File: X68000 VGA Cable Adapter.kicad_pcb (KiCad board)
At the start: 2 copper layers, 40.5 x 30.4 mm, 8 parts, among them J1 DE15_Receptacle_HighDensity, J2 DA15_Plug

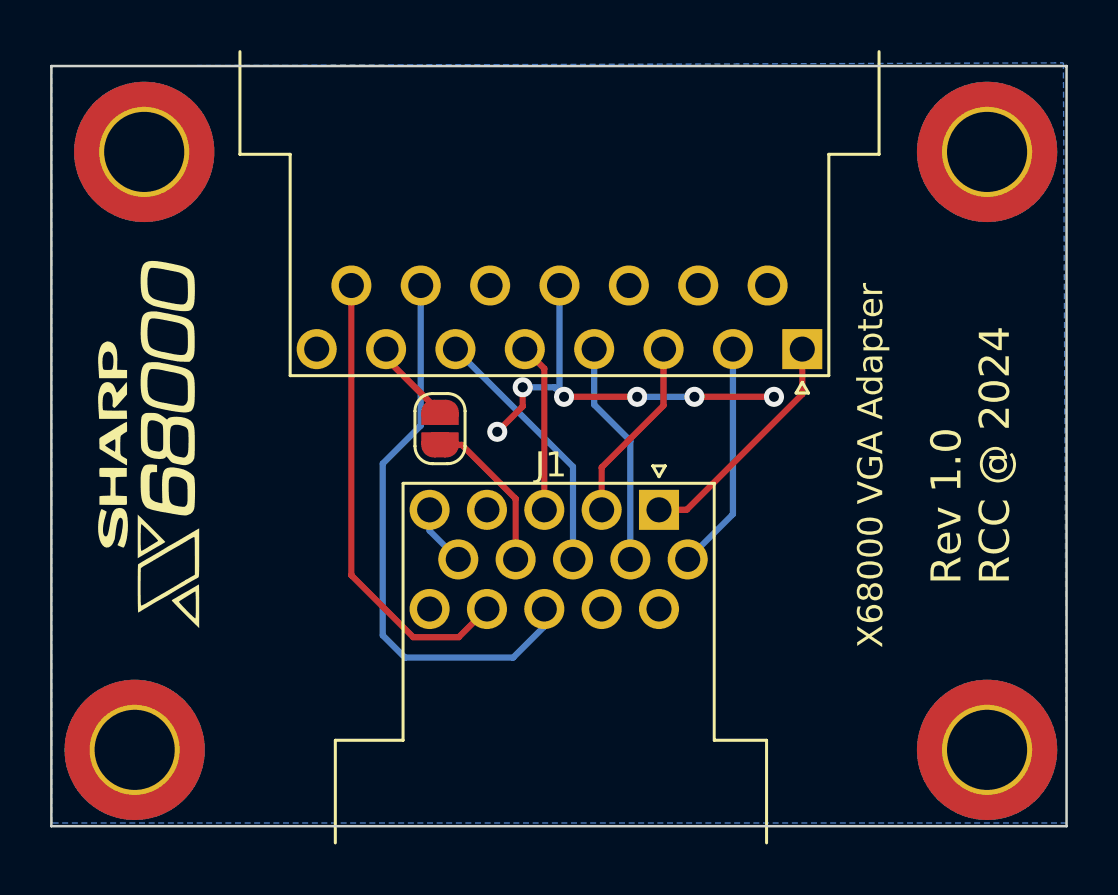
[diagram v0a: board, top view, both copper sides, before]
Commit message: Fabricated
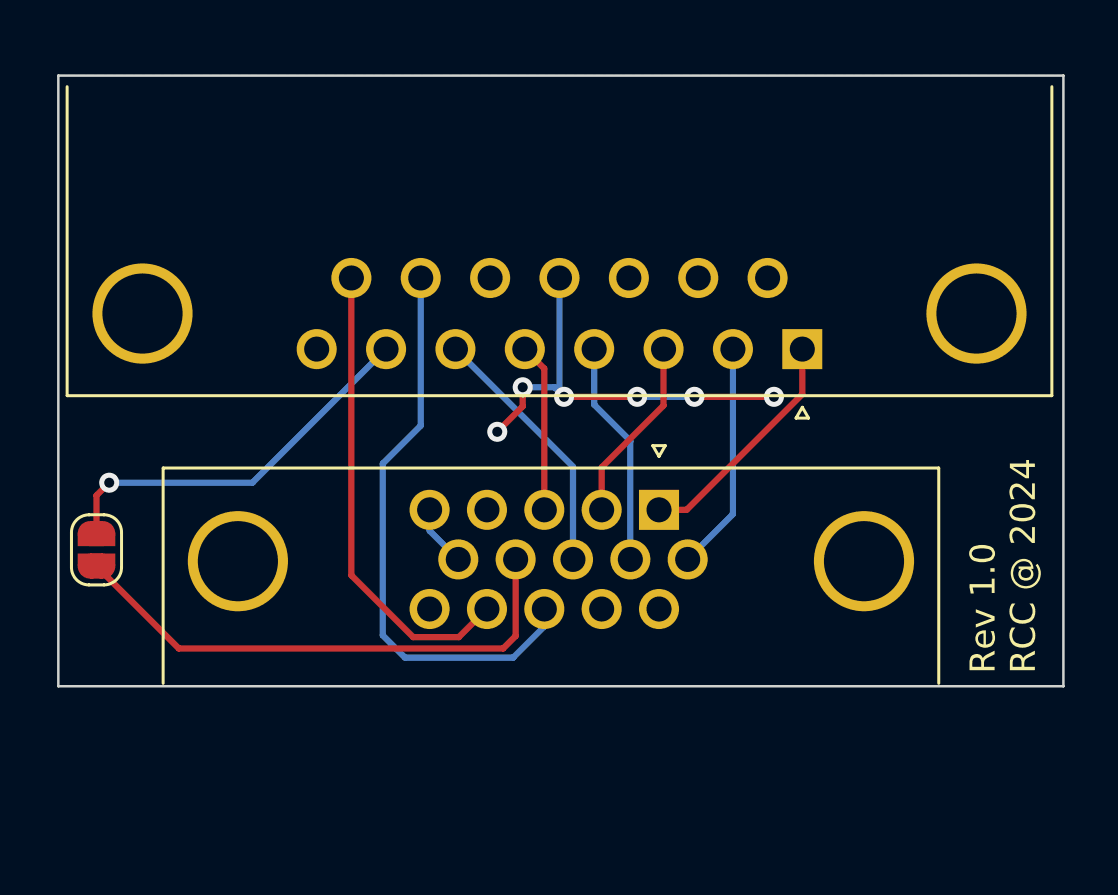
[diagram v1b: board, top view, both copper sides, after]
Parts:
- removed H1, H2, H3, H4: MountingHole, MountingHole:MountingHole_3.2mm_M3_DIN965_Pad_TopBottom
- G***: moved to B.Cu
- J1: footprint Connector_Dsub:DSUB-15-HD_Female_Horizontal_P2.29x1.98mm_EdgePinOffset9.40mm -> Connector_Dsub:DSUB-15-HD_Female_Horizontal_P2.29x1.98mm_EdgePinOffset3.03mm_Housed_MountingHolesOffset4.94mm
- J2: footprint Connector_Dsub:DSUB-15_Male_Horizontal_P2.77x2.54mm_EdgePinOffset9.40mm -> Connector_Dsub:DSUB-15_Male_Horizontal_P2.77x2.84mm_EdgePinOffset7.70mm_Housed_MountingHolesOffset9.12mm
- moved G*** 19.9 mm to (92.7, 51.9), turned to 180 degrees
- moved JP1 14.5 mm to (74.2, 67.2)
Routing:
- net VDC1: track 6.34 -> 21.4 mm
- net VDC2: track 3.42 -> 15.9 mm, vias 0 -> 1
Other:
- board size 40.5 x 30.4 mm -> 40.1 x 24.4 mm
- board text removed: "X68000 VGA Adapter"
